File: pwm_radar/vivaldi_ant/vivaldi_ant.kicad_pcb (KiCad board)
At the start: 2 copper layers, 34.1 x 20 mm, 1 part, among them J6 Conn_Coaxial

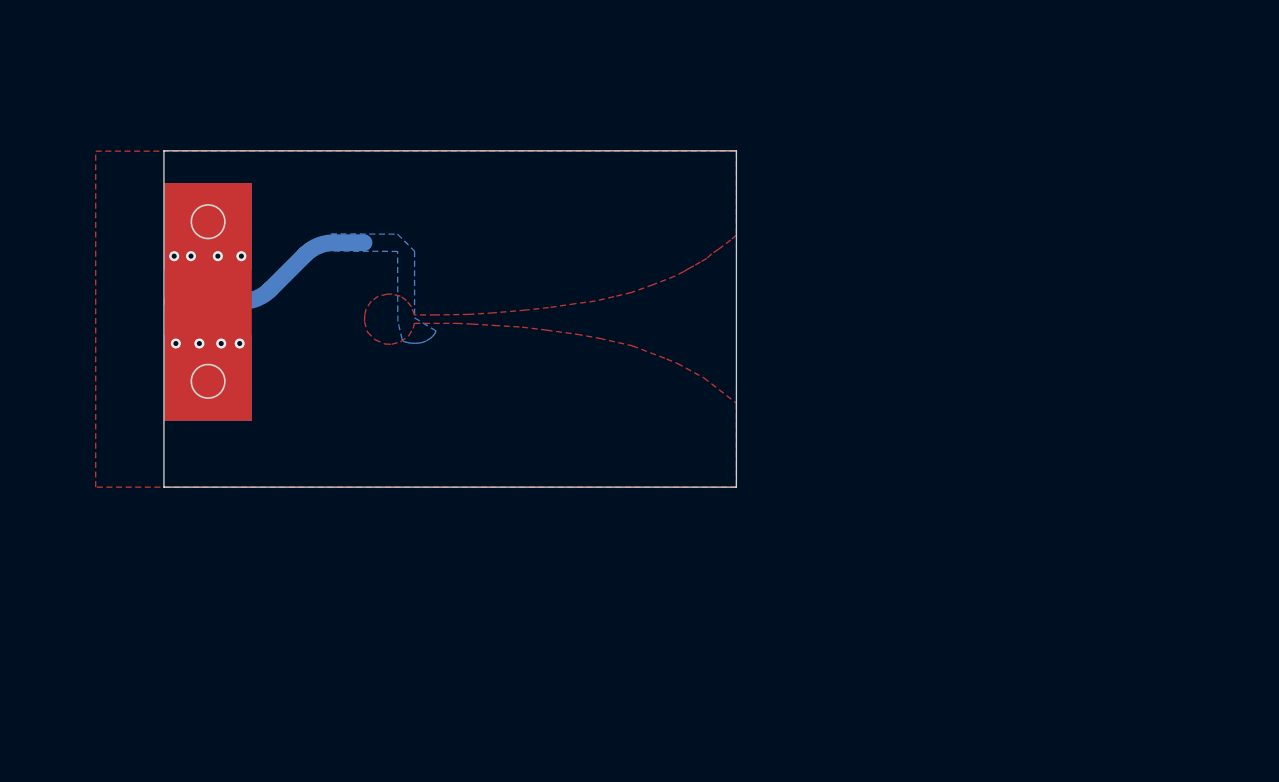
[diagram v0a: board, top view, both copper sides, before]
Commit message: fixing some final touches
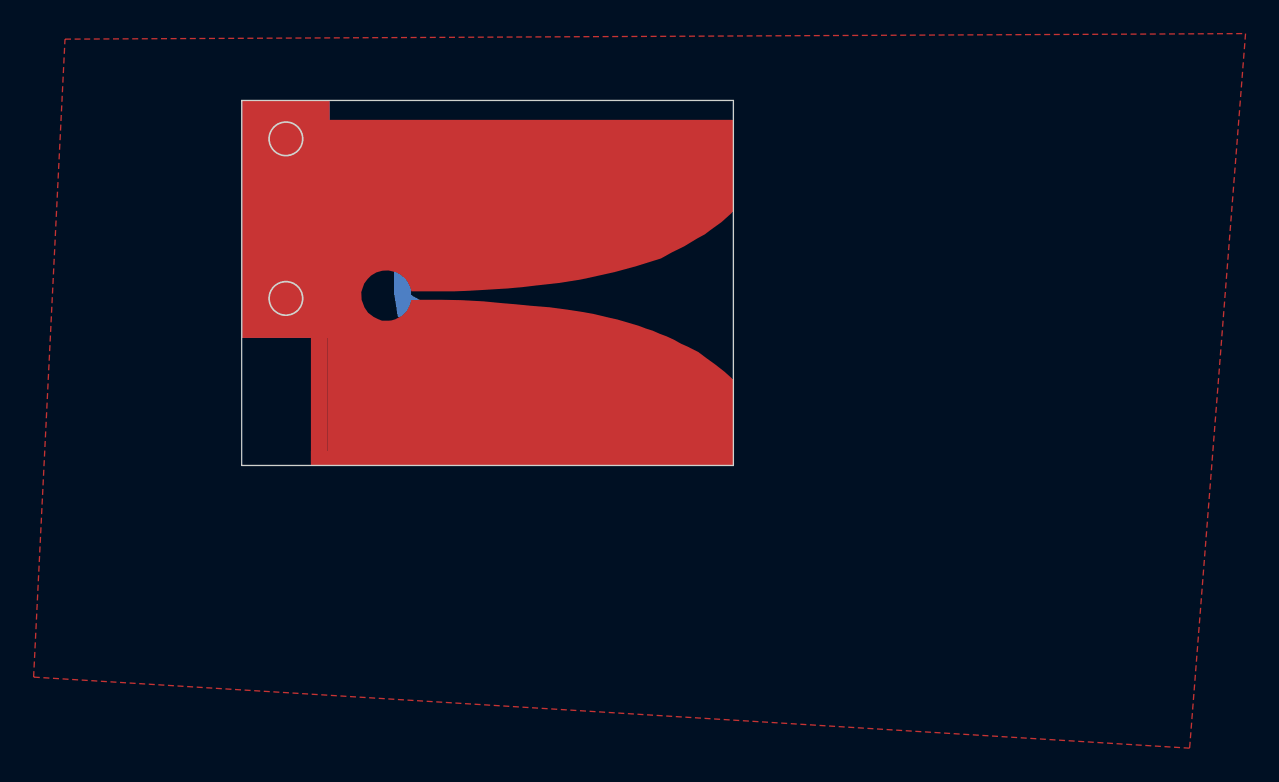
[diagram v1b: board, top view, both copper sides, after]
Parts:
- added U1: ~, RF_Antenna:Vivaldi Antenna 10 to 24 GHz, F.Cu at (130.2, 95.0)
- moved J6 6.77 mm to (136.2, 80.1)
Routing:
- net Net-(AE1-PCB_Trace): track 12.6 -> 0.00 mm
- net GND: vias 8 -> 0
- removed copper zone on B.Cu, net Net-(AE1-PCB_Trace)
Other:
- board size 34.1 x 20 mm -> 29.3 x 21.7 mm
